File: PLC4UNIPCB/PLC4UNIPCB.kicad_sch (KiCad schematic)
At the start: 4 parts, among them J1 Conn_01x09_Pin, J2 Conn_01x09_Pin, J3 Conn_01x09_Pin, J4 Conn_01x09_Pin

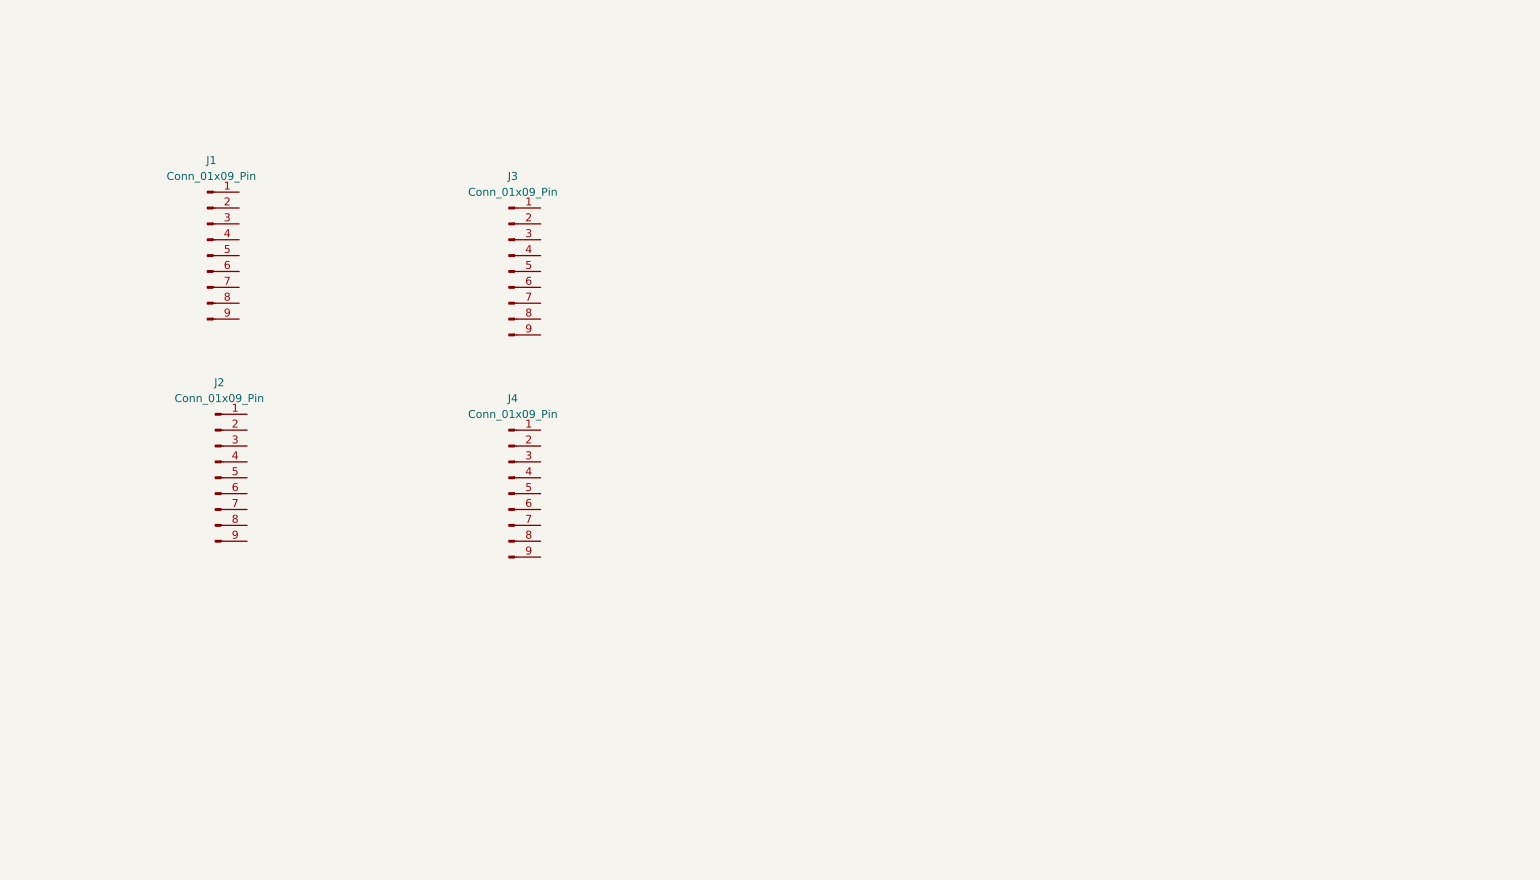
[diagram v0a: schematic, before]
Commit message: Add files via upload
Actualización de Esquemáticos
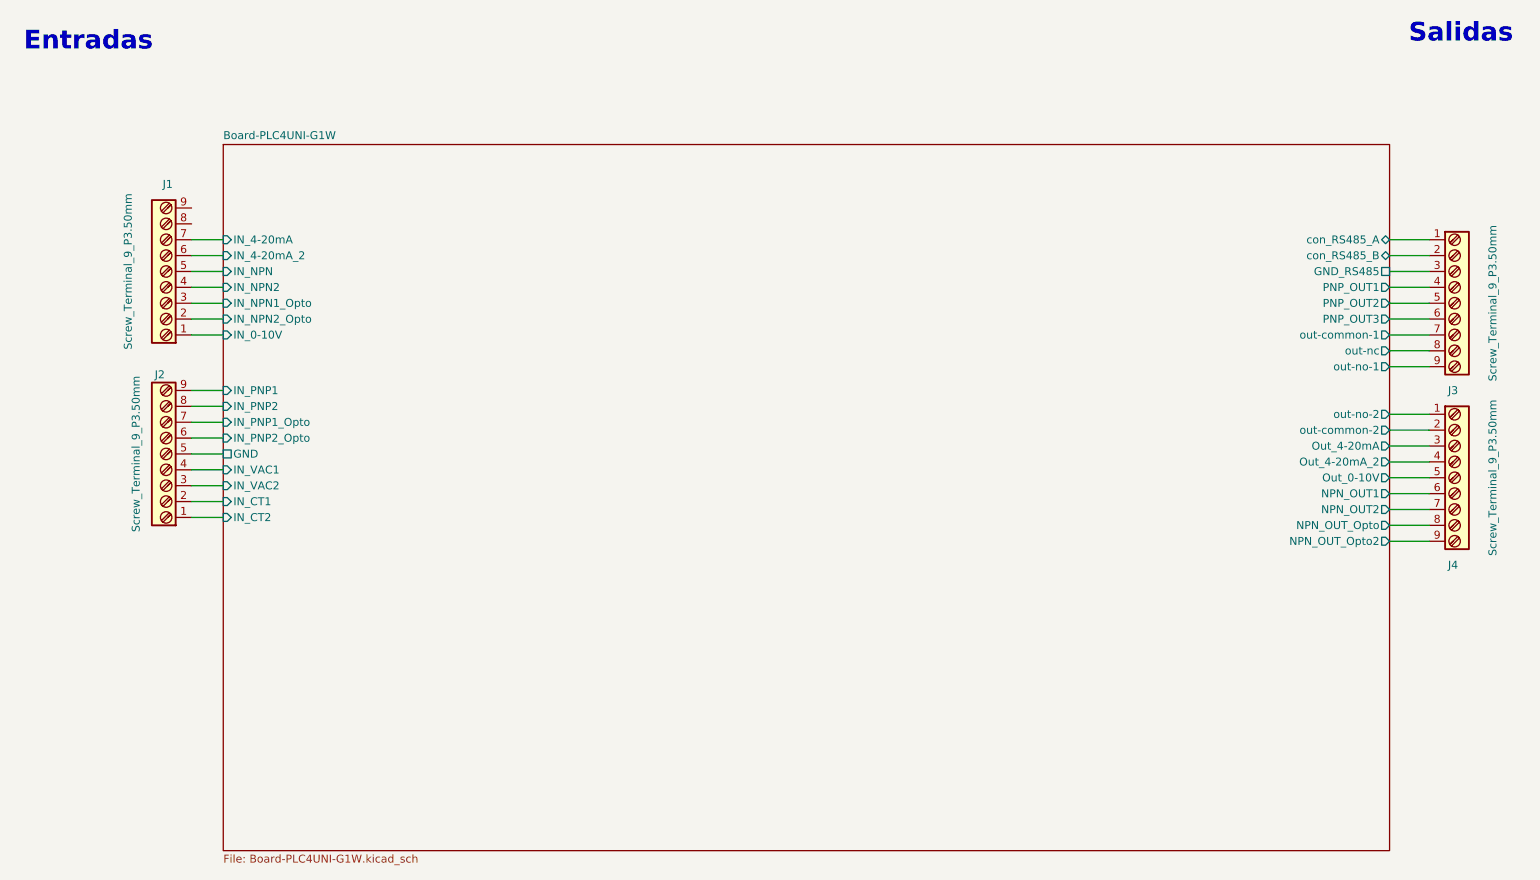
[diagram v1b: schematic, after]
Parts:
- removed J1, J2, J3, J4: Conn_01x09_Pin, symbol Connector:Conn_01x09_Pin
- added J1, J2, J3, J4: Screw_Terminal_9_P3.50mm, TerminalBlock_Phoenix:TerminalBlock_Phoenix_PT-1,5-9-3.5-H_1x09_P3.50mm_Horizontal, symbol GP8211S-TC50:Screw_Terminal_9_P3.50mm
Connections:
- new net Board-PLC4UNI-G1W/GND: J2.5
- new net Board-PLC4UNI-G1W/GND_RS485: J3.3
- new net Board-PLC4UNI-G1W/IN_0-10V: J1.1
- new net Board-PLC4UNI-G1W/IN_4-20mA: J1.7
- new net Board-PLC4UNI-G1W/IN_4-20mA_2: J1.6
- new net Board-PLC4UNI-G1W/IN_CT1: J2.2
- new net Board-PLC4UNI-G1W/IN_CT2: J2.1
- new net Board-PLC4UNI-G1W/IN_NPN: J1.5
- new net Board-PLC4UNI-G1W/IN_NPN1_Opto: J1.3
- new net Board-PLC4UNI-G1W/IN_NPN2: J1.4
- new net Board-PLC4UNI-G1W/IN_NPN2_Opto: J1.2
- new net Board-PLC4UNI-G1W/IN_PNP1: J2.9
- new net Board-PLC4UNI-G1W/IN_PNP1_Opto: J2.7
- new net Board-PLC4UNI-G1W/IN_PNP2: J2.8
- new net Board-PLC4UNI-G1W/IN_PNP2_Opto: J2.6
- new net Board-PLC4UNI-G1W/IN_VAC1: J2.4
- new net Board-PLC4UNI-G1W/IN_VAC2: J2.3
- new net Board-PLC4UNI-G1W/NPN_OUT1: J4.6
- new net Board-PLC4UNI-G1W/NPN_OUT2: J4.7
- new net Board-PLC4UNI-G1W/NPN_OUT_Opto: J4.8
- new net Board-PLC4UNI-G1W/NPN_OUT_Opto2: J4.9
- new net Board-PLC4UNI-G1W/Out_0-10V: J4.5
- new net Board-PLC4UNI-G1W/Out_4-20mA: J4.3
- new net Board-PLC4UNI-G1W/Out_4-20mA_2: J4.4
- new net Board-PLC4UNI-G1W/PNP_OUT1: J3.4
- new net Board-PLC4UNI-G1W/PNP_OUT2: J3.5
- new net Board-PLC4UNI-G1W/PNP_OUT3: J3.6
- new net Board-PLC4UNI-G1W/con_RS485_A: J3.1
- new net Board-PLC4UNI-G1W/con_RS485_B: J3.2
- new net Board-PLC4UNI-G1W/out-common-1: J3.7
- new net Board-PLC4UNI-G1W/out-common-2: J4.2
- new net Board-PLC4UNI-G1W/out-nc: J3.8
- new net Board-PLC4UNI-G1W/out-no-1: J3.9
- new net Board-PLC4UNI-G1W/out-no-2: J4.1
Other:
- added sheet Board-PLC4UNI-G1W (Board-PLC4UNI-G1W.kicad_sch)
- note added: "Entradas"
- note added: "Salidas"

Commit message: Add files via upload
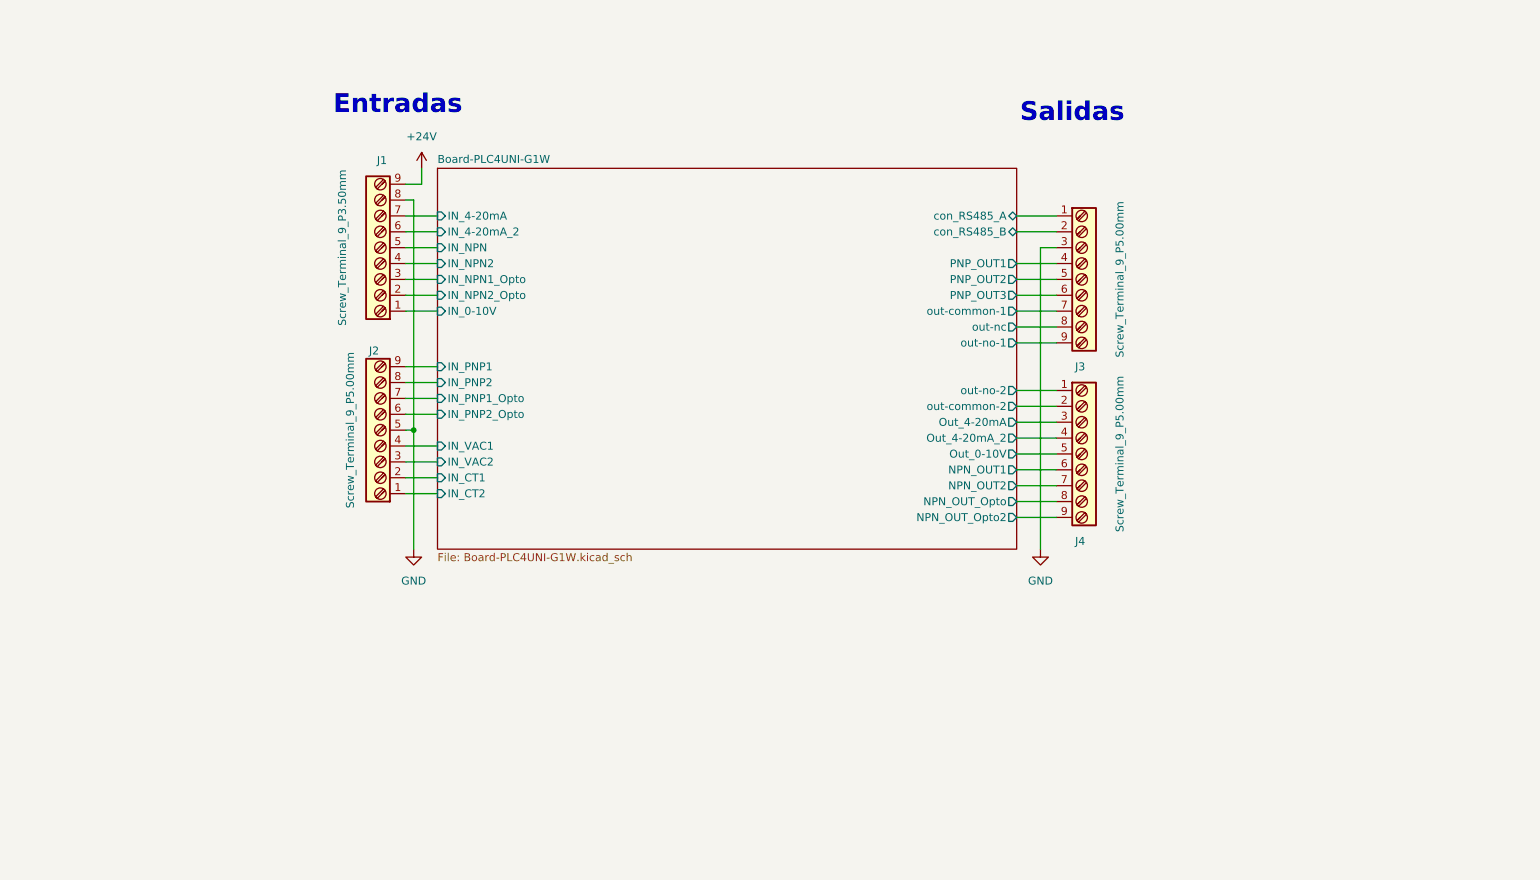
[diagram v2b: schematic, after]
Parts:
- J1: footprint TerminalBlock_Phoenix:TerminalBlock_Phoenix_PT-1,5-9-3.5-H_1x09_P3.50mm_Horizontal -> TerminalBlock_Phoenix:TerminalBlock_Phoenix_PT-1,5-9-5.0-H_1x09_P5.00mm_Horizontal
- J2, J3, J4: value Screw_Terminal_9_P3.50mm -> Screw_Terminal_9_P5.00mm; footprint TerminalBlock_Phoenix:TerminalBlock_Phoenix_PT-1,5-9-3.5-H_1x09_P3.50mm_Horizontal -> TerminalBlock_Phoenix:TerminalBlock_Phoenix_PT-1,5-9-5.0-H_1x09_P5.00mm_Horizontal
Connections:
- net Board-PLC4UNI-G1W/GND is gone; now on net GND: J2.5
- net Board-PLC4UNI-G1W/GND_RS485 is gone; now on net GND: J3.3
- net GND: now reaches J1.8
- net +24V: now reaches J1.9
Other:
- sheet Board-PLC4UNI-G1W ports: added none; removed GND, GND_RS485
- moved on the sheet: J1, J2, J3, J4
